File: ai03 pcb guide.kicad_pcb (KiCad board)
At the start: 2 copper layers, 77.8 x 38.1 mm, 24 parts, among them SW1 SW_Push, U1 ATmega32U4-AU, Y1 16MHz

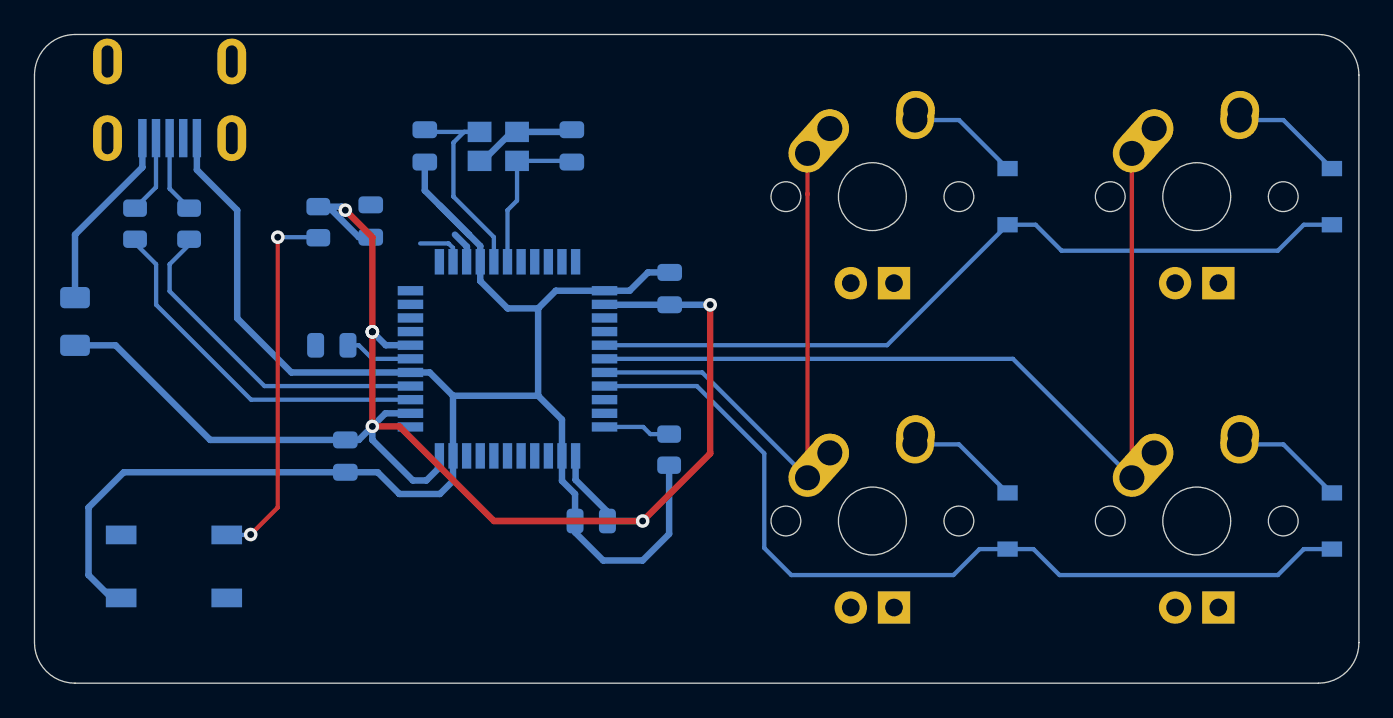
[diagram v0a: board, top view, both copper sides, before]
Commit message: added ground fill
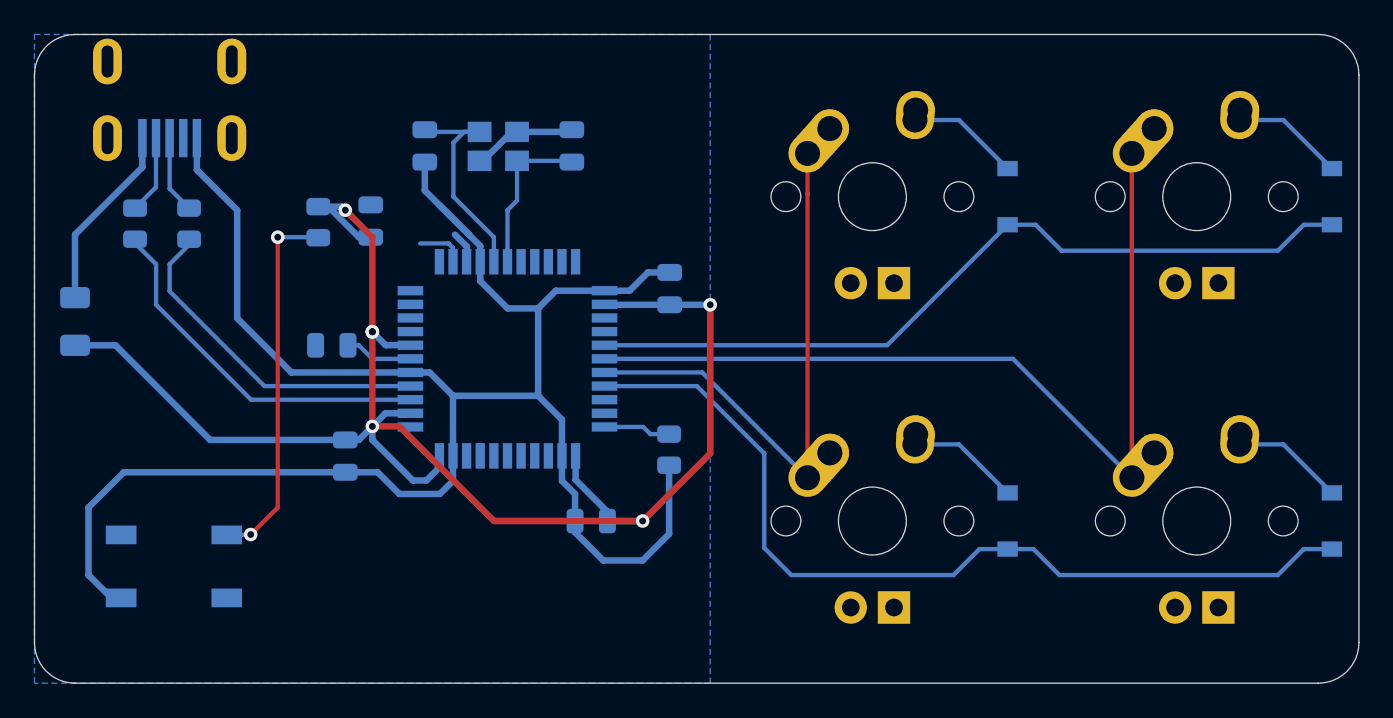
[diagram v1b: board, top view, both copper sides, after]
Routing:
- added copper zone on B.Cu, net GND
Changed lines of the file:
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@@
   (segment (start 75.4375 102.425) (end 73.16875 102.425) (width 0.254) (layer B.Cu) (net 20))
   (segment (start 75.859 102.8465) (end 75.4375 102.425) (width 0.254) (layer B.Cu) (net 20))
+  (zone (net 1) (net_name GND) (layer B.Cu) (hatch edge 0.508)
+    (connect_pads (clearance 0.508))
+    (min_thickness 0.254)
+    (fill yes (arc_segments 32) (thermal_gap 0.508) (thermal_bridge_width 0.508))
+    (polygon
+      (pts
+        (xy 79.375 117.475) (xy 39.6875 117.475) (xy 39.6875 79.375) (xy 79.375 79.375)
+      )
+    )
+  )
 )
